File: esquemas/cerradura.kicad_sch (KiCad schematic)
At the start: 2 parts, among them J1 Conn_02x20_Odd_Even, J2 Conn_02x20_Odd_Even

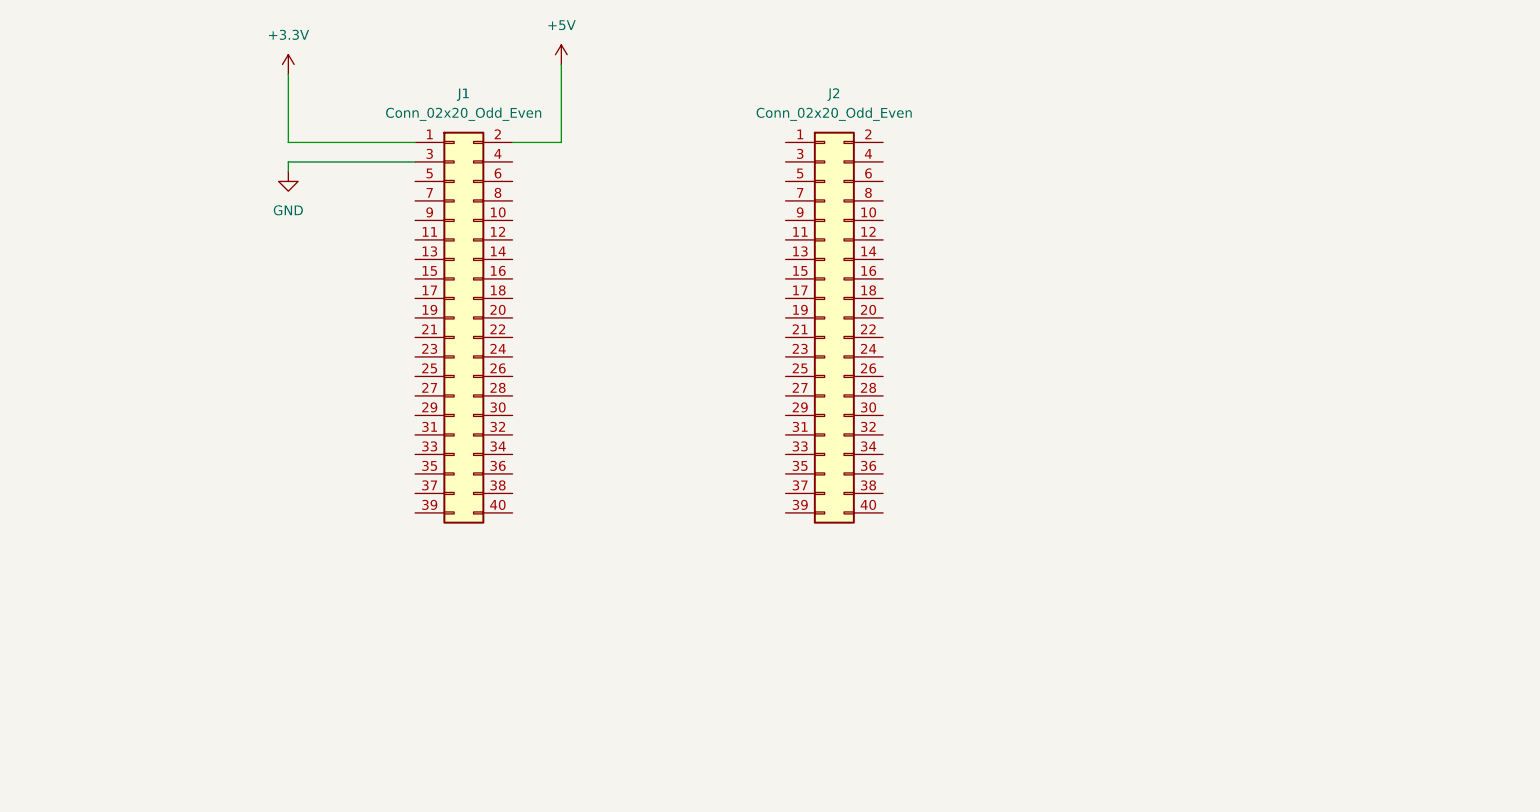
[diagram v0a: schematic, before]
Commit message: update
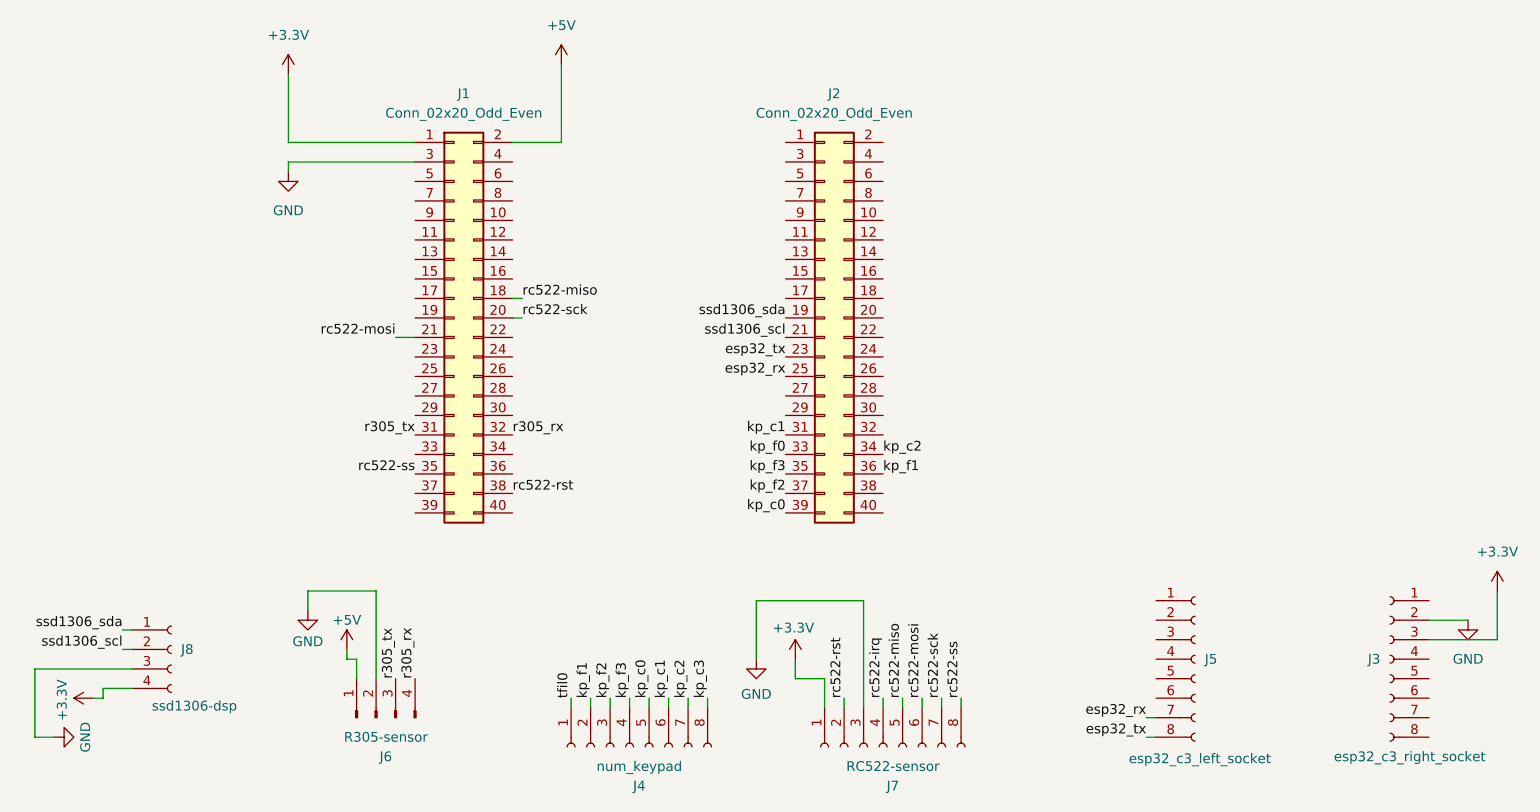
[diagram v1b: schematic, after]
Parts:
- added J3: esp32_c3_right_socket, Connector_Harwin:Harwin_M20-89008xx_1x08_P2.54mm_Horizontal, symbol Connector:Conn_01x08_Socket
- added J4: num_keypad, Connector_Harwin:Harwin_M20-89008xx_1x08_P2.54mm_Horizontal, symbol Connector:Conn_01x08_Socket
- added J5: esp32_c3_left_socket, Connector_Harwin:Harwin_M20-89008xx_1x08_P2.54mm_Horizontal, symbol Connector:Conn_01x08_Socket
- added J6: R305-sensor, Connector:FanPinHeader_1x04_P2.54mm_Vertical, symbol Connector:Conn_01x04_Pin
- added J7: RC522-sensor, Connector_Harwin:Harwin_M20-89008xx_1x08_P2.54mm_Horizontal, symbol Connector:Conn_01x08_Socket
- added J8: ssd1306-dsp, Connector_Harwin:Harwin_M20-89004xx_1x04_P2.54mm_Horizontal, symbol Connector:Conn_01x04_Socket
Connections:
- net +3.3V: now also J3.3 (Pin_3), J7.1 (Pin_1), J8.4 (Pin_4)
- net +5V: now also J6.1 (Pin_1)
- net GND: now also J3.2 (Pin_2), J6.2 (Pin_2), J7.3 (Pin_3), J8.3 (Pin_3)
- net ssd1306_sda: now reaches J2.19 (Pin_19)
- net ssd1306_sda: now also J8.1 (Pin_1)
- net ssd1306_scl: now reaches J2.21 (Pin_21)
- net ssd1306_scl: now also J8.2 (Pin_2)
- net esp32_tx: now reaches J2.23 (Pin_23)
- net esp32_tx: now also J5.8 (Pin_8)
- net esp32_rx: now reaches J2.25 (Pin_25)
- net esp32_rx: now also J5.7 (Pin_7)
- net kp_c1: now reaches J2.31 (Pin_31)
- net kp_c1: now also J4.6 (Pin_6)
- net kp_f0: now reaches J2.33 (Pin_33)
- net kp_c2: now reaches J2.34 (Pin_34)
- net kp_c2: now also J4.7 (Pin_7)
- net kp_f3: now reaches J2.35 (Pin_35)
- net kp_f3: now also J4.4 (Pin_4)
- net kp_f1: now reaches J2.36 (Pin_36)
- net kp_f1: now also J4.2 (Pin_2)
- net kp_f2: now reaches J2.37 (Pin_37)
- net kp_f2: now also J4.3 (Pin_3)
- net kp_c0: now reaches J2.39 (Pin_39)
- net kp_c0: now also J4.5 (Pin_5)
- net rc522-miso: now reaches J1.18 (Pin_18)
- net rc522-miso: now also J7.5 (Pin_5)
- net rc522-sck: now reaches J1.20 (Pin_20)
- net rc522-sck: now also J7.7 (Pin_7)
- net rc522-mosi: now reaches J1.21 (Pin_21)
- net rc522-mosi: now also J7.6 (Pin_6)
- net r305_tx: now reaches J1.31 (Pin_31)
- net r305_tx: now also J6.3 (Pin_3)
- net r305_rx: now reaches J1.32 (Pin_32)
- net r305_rx: now also J6.4 (Pin_4)
- net rc522-ss: now reaches J1.35 (Pin_35)
- net rc522-ss: now also J7.8 (Pin_8)
- net rc522-rst: now reaches J1.38 (Pin_38)
- net rc522-rst: now also J7.2 (Pin_2)
- new net kp_c3: J4.8 (Pin_8)
- new net rc522-irq: J7.4 (Pin_4)
- new net tfil0: J4.1 (Pin_1)
